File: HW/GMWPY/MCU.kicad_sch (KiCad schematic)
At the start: 33 parts, among them J3 Conn_01x10, J4 Micro_SD_Card_Det, SW1 MCU_RESET, SW2 MCU_RESET, U14 ESP32-S3-WROOM-1

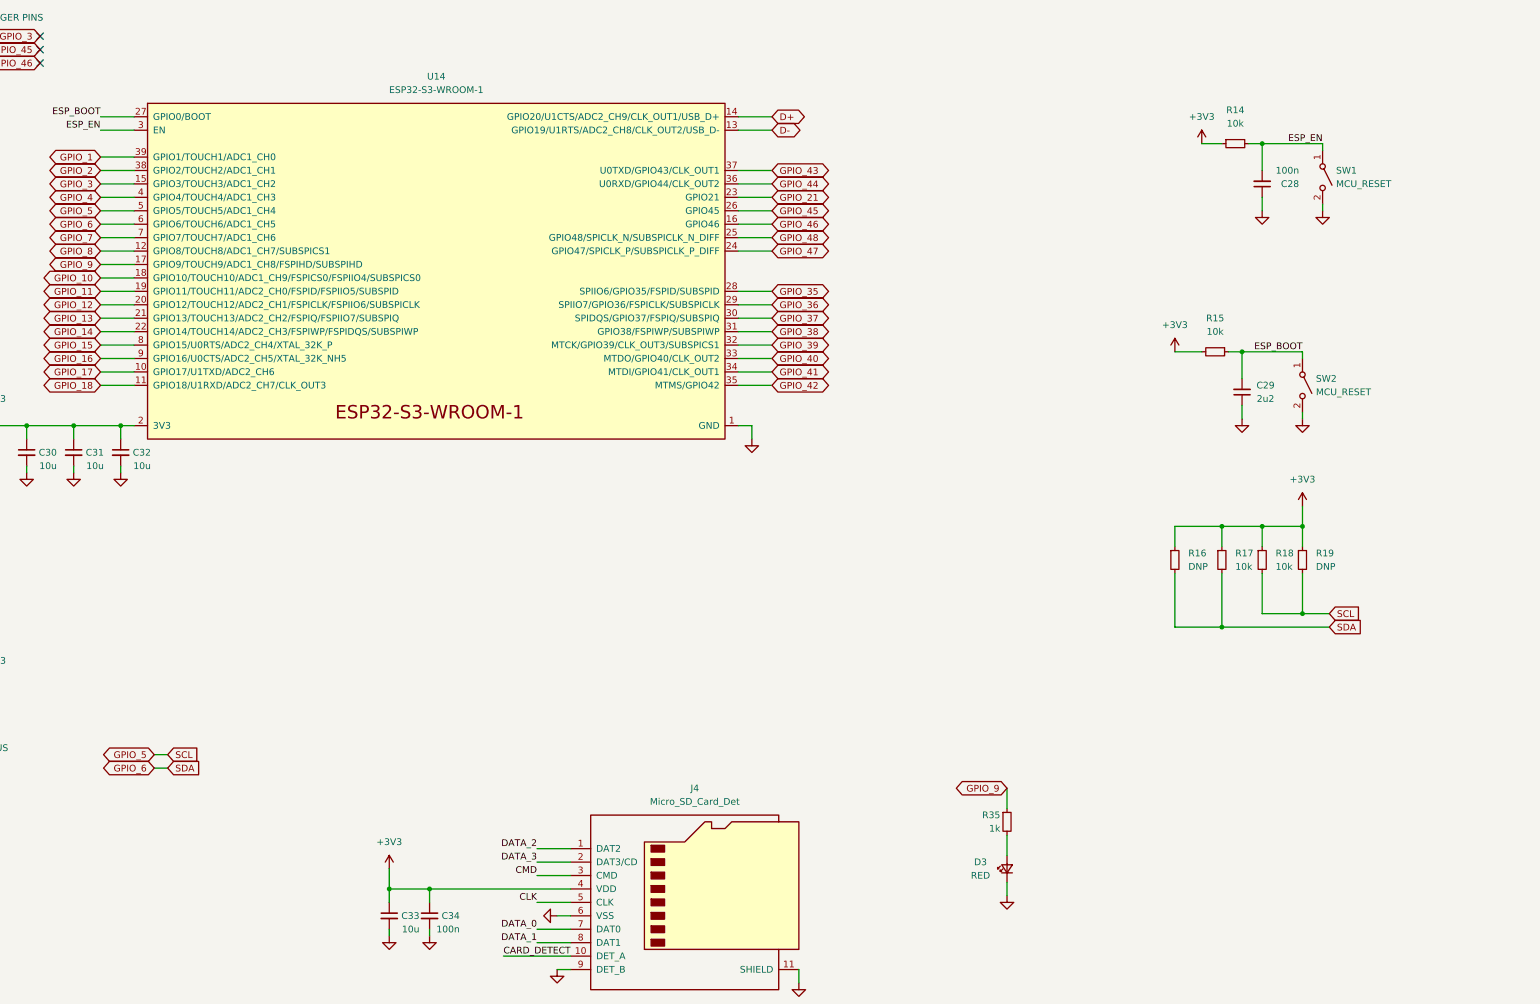
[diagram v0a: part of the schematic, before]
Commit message: f
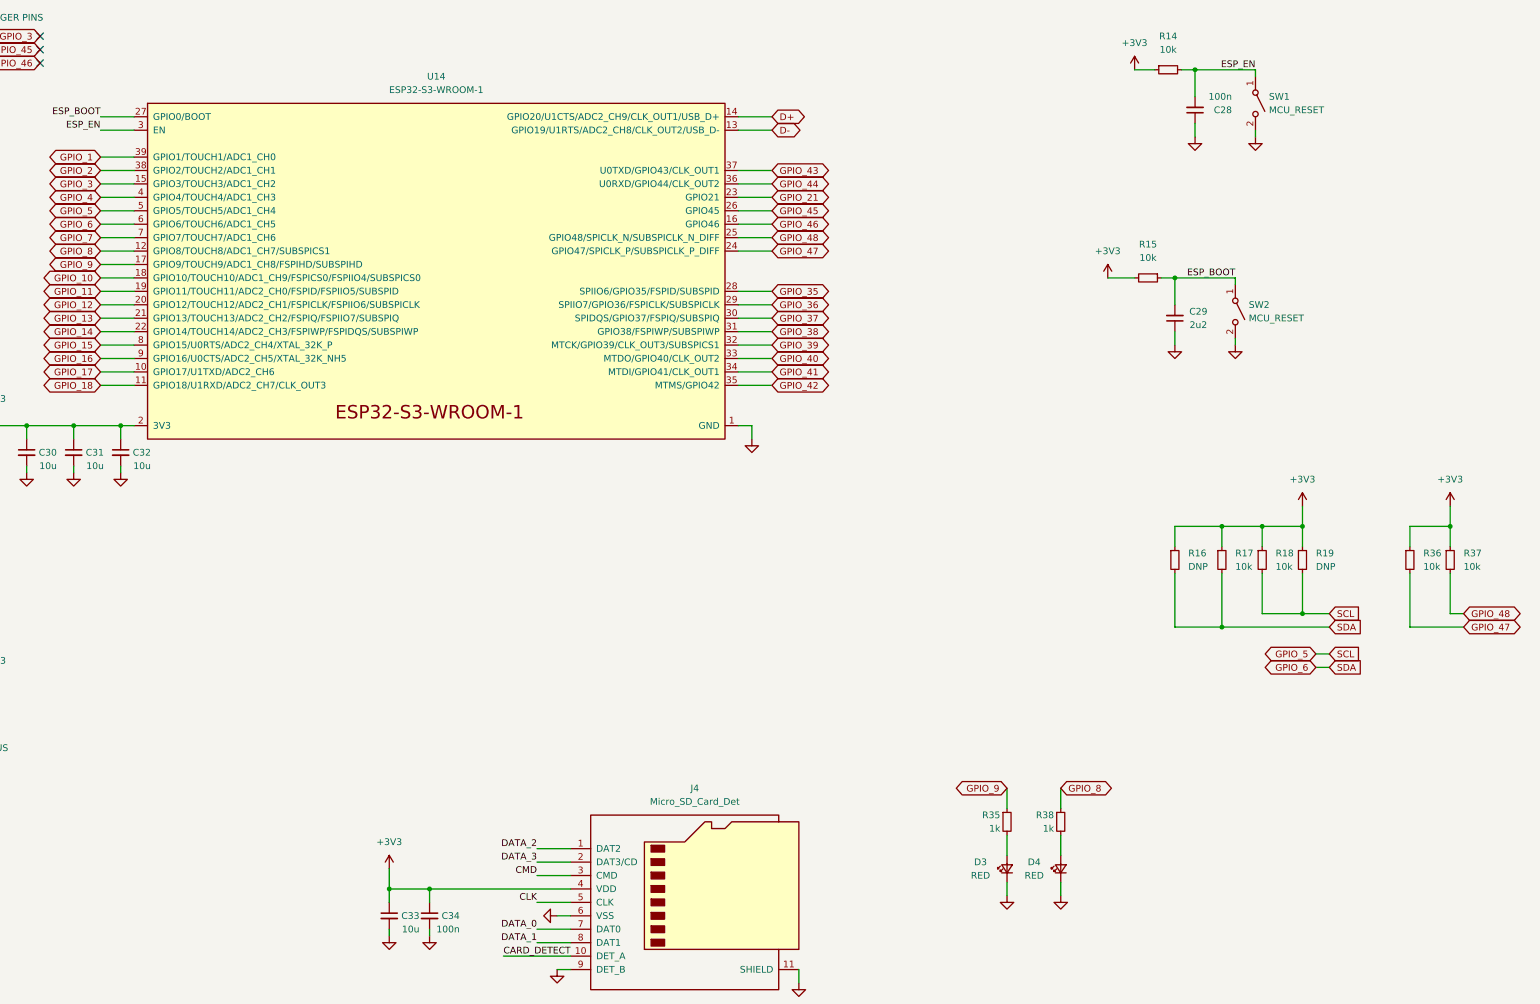
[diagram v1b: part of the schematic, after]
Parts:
- added D4: RED, LED_SMD:LED_0603_1608Metric, symbol Device:LED_Small
- added R36, R37: 10k, Resistor_SMD:R_0603_1608Metric_Pad0.98x0.95mm_HandSolder, symbol Device:R_Small
- added R38: 1k, Resistor_SMD:R_0603_1608Metric, symbol Device:R_Small
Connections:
- net +3V3: now also R36.1, R37.1
- net GND: now also D4.1 (K)
- net GPIO_47: now also R36.2
- net GPIO_48: now also R37.2
- net GPIO_8: now also R38.1
- new net: D4.2 (A), R38.2
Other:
- moved on the sheet: C28, C29, R14, R15, SW1, SW2

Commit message: f
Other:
- note added: "MCU"
- note added: "Pull UPs"
- note added: "SD card"
- moved on the sheet: C28, C29, C30, C31, C32, C33, C34, D3, D4, J3, J4, R14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
